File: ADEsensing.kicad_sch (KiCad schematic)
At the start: 4 parts, among them IC1 ISO6762DWR, IC2 TPS7A2425DBVR, U5 ADE7953xCP, Y2 ABLS-3.579545MHZ-B4-T

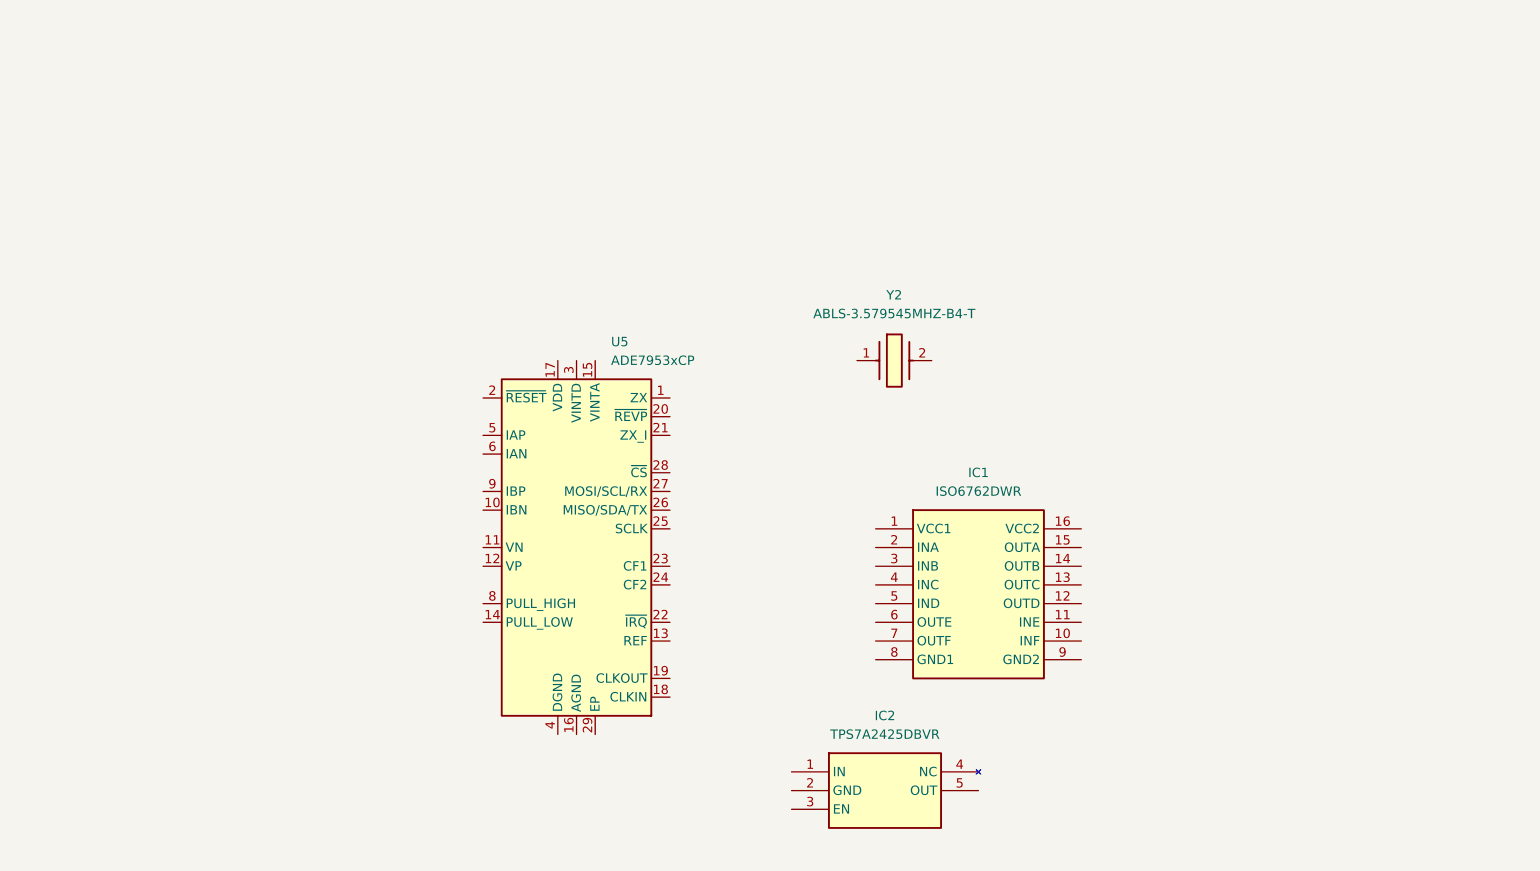
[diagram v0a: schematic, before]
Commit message: ade7953 breakout board
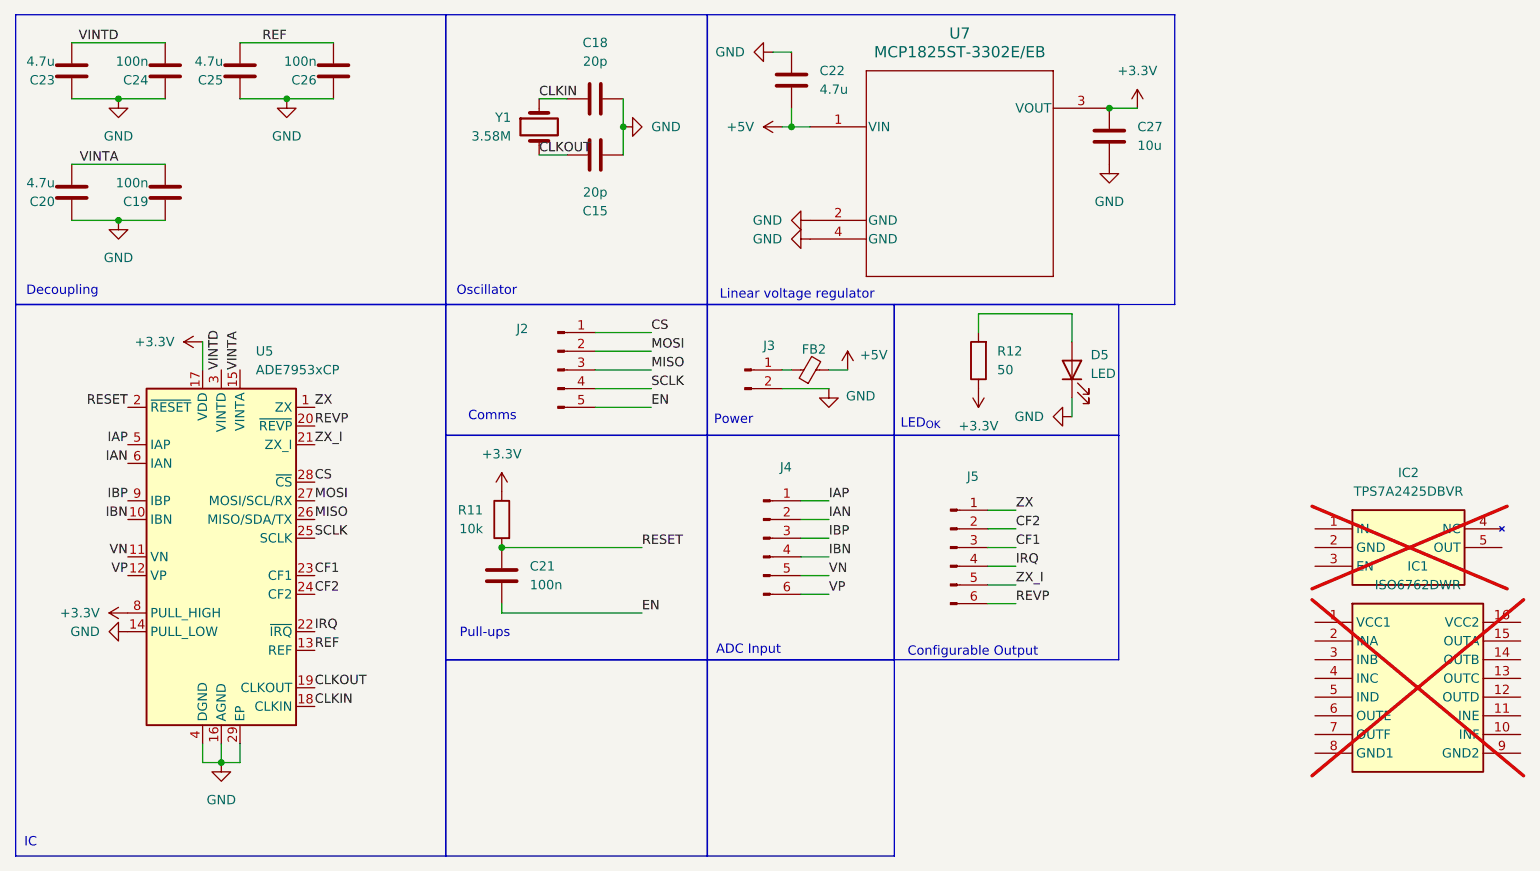
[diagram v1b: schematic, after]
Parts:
- removed Y2: ABLS-3.579545MHZ-B4-T, ABLS3579545MHZB4T, symbol SamacSys_Parts:ABLS-3.579545MHZ-B4-T
- added C15, C18: 20p, Capacitor_SMD:C_0603_1608Metric, symbol Device:C
- added C19, C21, C24, C26: 100n, Capacitor_SMD:C_0603_1608Metric, symbol Device:C
- added C20, C22, C23, C25: 4.7u, Capacitor_SMD:C_0805_2012Metric, symbol Device:C
- added C27: 10u, Capacitor_SMD:C_0805_2012Metric, symbol Device:C
- added D5: LED, LED_SMD:LED_0805_2012Metric, symbol Device:LED
- added FB2: FerriteBead_Small, Inductor_SMD:L_0805_2012Metric, symbol Device:FerriteBead_Small
- added J2: Conn_01x05_Pin, Connector_PinHeader_2.54mm:PinHeader_1x05_P2.54mm_Vertical, symbol Connector:Conn_01x05_Pin
- added J3: Conn_01x02_Pin, Connector_PinHeader_2.54mm:PinHeader_1x02_P2.54mm_Vertical, symbol Connector:Conn_01x02_Pin
- added J4, J5: Conn_01x06_Pin, Connector_PinHeader_2.54mm:PinHeader_1x06_P2.54mm_Vertical, symbol Connector:Conn_01x06_Pin
- added R11: 10k, Resistor_SMD:R_0805_2012Metric, symbol Device:R
- added R12: 50, Resistor_SMD:R_0805_2012Metric, symbol Device:R
- added U7: MCP1825ST-3302E/EB, SmartSupplyLib:DDPAK3_MC_MCH, symbol SmartSupplyLib:MCP1825ST-3302E_EB
- added Y1: 3.58M, Crystal:Crystal_SMD_HC49-SD, symbol Device:Crystal
- IC1, IC2: now not fitted; now left out of the parts list
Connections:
- net ZX: now reaches U5.1 (ZX)
- net ZX: now also J5.1 (Pin_1)
- net IBN: now reaches U5.10 (IBN)
- net IBN: now also J4.4 (Pin_4)
- net VN: now reaches U5.11 (VN)
- net VN: now also J4.5 (Pin_5)
- net VP: now reaches U5.12 (VP)
- net VP: now also J4.6 (Pin_6)
- net REF: now reaches U5.13 (REF)
- net REF: now also C25.2, C26.2
- net GND: now reaches U5.14 (PULL_LOW)
- net GND: now also U5.16 (AGND), U5.29 (EP), U5.4 (DGND), C15.1, C18.2, C19.1, C20.1, C22.1, C23.1, C24.1, C25.1, C26.1, C27.2, D5.1 (K), J3.2 (Pin_2), U7.2 (GND), U7.4 (GND)
- net VINTA: now reaches U5.15 (VINTA)
- net VINTA: now also C19.2, C20.2
- net +3.3V: now reaches U5.17 (VDD)
- net +3.3V: now also U5.7 (PULL_HIGH), U5.8 (PULL_HIGH), C27.1, R11.1, R12.1, U7.3 (VOUT)
- net CLKIN: now reaches U5.18 (CLKIN)
- net CLKIN: now also C18.1, Y1.1
- net CLKOUT: now reaches U5.19 (CLKOUT)
- net CLKOUT: now also C15.2, Y1.2
- net RESET: now reaches U5.2 (~{RESET})
- net RESET: now also C21.1, R11.2
- net REVP: now reaches U5.20 (~{REVP})
- net REVP: now also J5.6 (Pin_6)
- net ZX_I: now reaches U5.21 (ZX_I)
- net ZX_I: now also J5.5 (Pin_5)
- net IRQ: now reaches U5.22 (~{IRQ})
- net IRQ: now also J5.4 (Pin_4)
- net CF1: now reaches U5.23 (CF1)
- net CF1: now also J5.3 (Pin_3)
- net CF2: now reaches U5.24 (CF2)
- net CF2: now also J5.2 (Pin_2)
- net SCLK: now reaches U5.25 (SCLK)
- net SCLK: now also J2.4 (Pin_4)
- net MISO: now reaches U5.26 (MISO/SDA/TX)
- net MISO: now also J2.3 (Pin_3)
- net MOSI: now reaches U5.27 (MOSI/SCL/RX)
- net MOSI: now also J2.2 (Pin_2)
- net CS: now reaches U5.28 (~{CS})
- net CS: now also J2.1 (Pin_1)
- net VINTD: now reaches U5.3 (VINTD)
- net VINTD: now also C23.2, C24.2
- net IAP: now reaches U5.5 (IAP)
- net IAP: now also J4.1 (Pin_1)
- net IAN: now reaches U5.6 (IAN)
- net IAN: now also J4.2 (Pin_2)
- net IBP: now reaches U5.9 (IBP)
- net IBP: now also J4.3 (Pin_3)
- new net: D5.2 (A), R12.2
- new net: FB2.1, J3.1 (Pin_1)
- new net +5V: C22.2, FB2.2, U7.1 (VIN)
- new net EN: C21.2, J2.5 (Pin_5)
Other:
- note added: "ADC Input"
- note added: "Comms"
- note added: "Configurable Output"
- note added: "Decoupling"
- note added: "IC"
- note added: "LED_{OK}"
- note added: "Linear voltage regulator"
- note added: "Oscillator"
- note added: "Power"
- note added: "Pull-ups"
- moved on the sheet: U5
